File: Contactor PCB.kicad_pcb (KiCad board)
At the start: 2 copper layers, 140.5 x 83.8 mm, 29 parts, among them J1 TSCU, J10 COIL2_CONNECTOR, J11 AUX2_CONNECTOR, J2 TSCU, J3 IMD, J4 AIL, J5 UIL, J6 TBD, J7 COIL_INPUTS, J8 COIL1_CONNECTOR, J9 AUX1_CONNECTOR, U1 Gigavac_GX21CAB, U2 Gigavac_GX21CAB

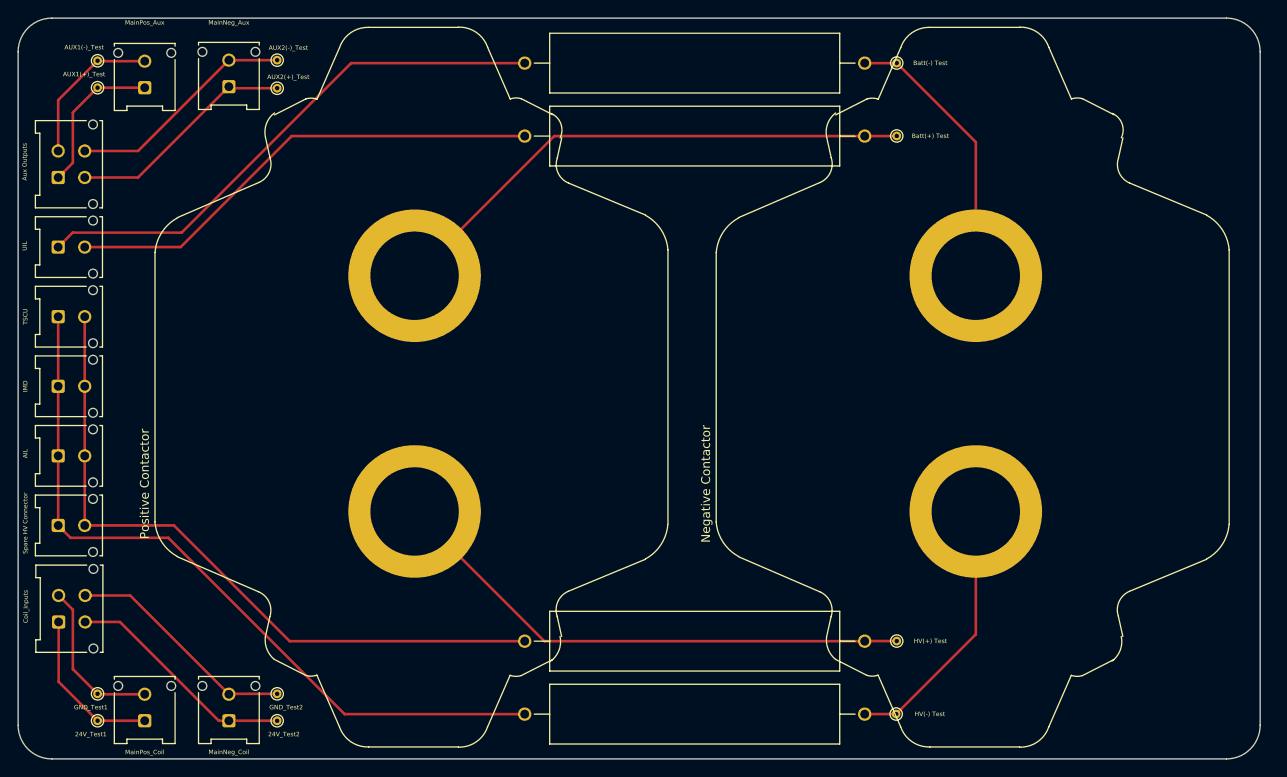
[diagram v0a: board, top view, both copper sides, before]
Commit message: Finalize Board
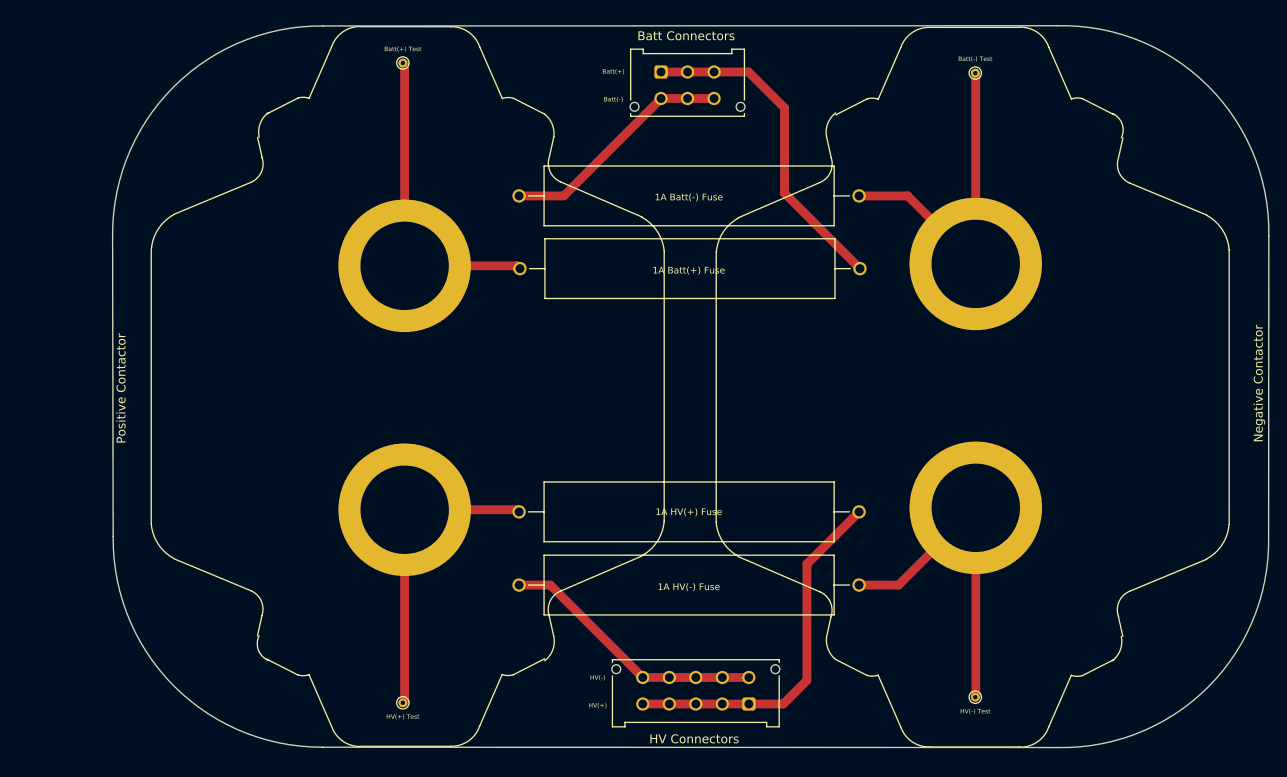
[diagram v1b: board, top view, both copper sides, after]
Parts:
- removed J10: COIL2_CONNECTOR, Connector_Molex:Molex_Micro-Fit_3.0_43045-0212_2x01_P3.00mm_Vertical
- removed J11: AUX2_CONNECTOR, Connector_Molex:Molex_Micro-Fit_3.0_43045-0212_2x01_P3.00mm_Vertical
- removed J3: IMD, Connector_Molex:Molex_Micro-Fit_3.0_43045-0212_2x01_P3.00mm_Vertical
- removed J4: AIL, Connector_Molex:Molex_Micro-Fit_3.0_43045-0212_2x01_P3.00mm_Vertical
- removed J5: UIL, Connector_Molex:Molex_Micro-Fit_3.0_43045-0212_2x01_P3.00mm_Vertical
- removed J6: TBD, Connector_Molex:Molex_Micro-Fit_3.0_43045-0212_2x01_P3.00mm_Vertical
- removed J7: COIL_INPUTS, Connector_Molex:Molex_Micro-Fit_3.0_43045-0412_2x02_P3.00mm_Vertical
- removed J8: COIL1_CONNECTOR, Connector_Molex:Molex_Micro-Fit_3.0_43045-0212_2x01_P3.00mm_Vertical
- removed J9: AUX1_CONNECTOR, Connector_Molex:Molex_Micro-Fit_3.0_43045-0212_2x01_P3.00mm_Vertical
- removed TP10: 24V_TEST2, TestPoint:TestPoint_THTPad_D1.0mm_Drill0.5mm
- removed TP11: GND_TEST1, TestPoint:TestPoint_THTPad_D1.0mm_Drill0.5mm
- removed TP12: 24V_TEST1, TestPoint:TestPoint_THTPad_D1.0mm_Drill0.5mm
- removed TP2, TP6: AUX_TEST(+), TestPoint:TestPoint_THTPad_D1.0mm_Drill0.5mm
- removed TP3, TP7: AUX_TEST(-), TestPoint:TestPoint_THTPad_D1.0mm_Drill0.5mm
- removed TP9: GND_TEST2, TestPoint:TestPoint_THTPad_D1.0mm_Drill0.5mm
- F1, F2, F3, F4: footprint CustomFootprints:Fuse_Placeholder -> CustomFootprints:0ADAP1000RE
- J1: value TSCU -> HV Connector; footprint Connector_Molex:Molex_Micro-Fit_3.0_43045-0212_2x01_P3.00mm_Vertical -> Connector_Molex:Molex_Micro-Fit_3.0_43045-1012_2x05_P3.00mm_Vertical
- J2: value TSCU -> Batt Connector; footprint Connector_Molex:Molex_Micro-Fit_3.0_43045-0412_2x02_P3.00mm_Vertical -> Connector_Molex:Molex_Micro-Fit_3.0_43045-0612_2x03_P3.00mm_Vertical
- moved U1 100.1 mm to (176.9, 44.0), turned to -90 degrees
- moved J1 89.6 mm to (186.5, 120.8), turned to 180 degrees
- moved J2 69.2 mm to (176.5, 49.3), turned to 0 degrees
- moved TP1 56.5 mm to (147.3, 48.3)
- moved TP4 56.3 mm to (147.3, 120.7)
- moved F2 29.0 mm to (179.6, 91.9), turned to 0 degrees
- moved F3 15.0 mm to (179.8, 70.5)
- moved F4 14.6 mm to (179.8, 114.5)
- moved TP8 9.16 mm to (212.1, 120.0)
- moved TP5 8.96 mm to (212.1, 49.4)
- moved F1 0.96 mm to (179.7, 64.3), turned to 0 degrees
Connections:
- F1 pad 1: Net-(F1-Pad1) -> Net-(U1-Pad1)
- F2 pad 1: Net-(F2-Pad1) -> Net-(TP4-Pad1)
- J1 pad 1: /HV(-) -> /HV(+)
- J2 pad 1: /AUX_1(+) -> /Batt(+)
- J2 pad 2: /AUX_1(-) -> /Batt(+)
- J2 pad 3: /AUX_2(+) -> /Batt(+)
- J2 pad 4: /AUX_2(-) -> /Batt(-)
- TP1 pad 1: Net-(F1-Pad1) -> Net-(U1-Pad1)
- TP4 pad 1: Net-(F2-Pad1) -> Net-(TP4-Pad1)
- U1 pad 1: Net-(F2-Pad1) -> Net-(U1-Pad1)
- U1 pad 2: Net-(F1-Pad1) -> Net-(TP4-Pad1)
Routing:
- net Net-(F1-Pad1): track 61.1 -> 0.00 mm
- net Net-(F2-Pad1): track 60.6 -> 0.00 mm
- net /HV(-): track 85.2 -> 30.3 mm
- net /HV(+): track 78.8 -> 41.2 mm
- net Net-(U1-Pad1): track 0.00 -> 36.2 mm
- net Net-(TP4-Pad1): track 0.00 -> 35.0 mm
- net /Batt(-): track 61.4 -> 26.6 mm
- net /GND_2: track 26.4 -> 0.00 mm
- net /24V_IN2: track 26.4 -> 0.00 mm
- net /AUX_2(+): track 26.1 -> 0.00 mm
- net /AUX_2(-): track 26.0 -> 0.00 mm
- net /24V_IN1: track 18.3 -> 0.00 mm
- net /GND_1: track 18.3 -> 0.00 mm
- net /Batt(+): track 55.0 -> 37.4 mm
- net /AUX_1(-): track 17.4 -> 0.00 mm
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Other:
- board size 140.5 x 83.8 mm -> 130.8 x 81.7 mm
- board text added: "1A Batt(+) Fuse"
- board text added: "1A Batt(-) Fuse"
- board text added: "1A HV(+) Fuse"
- board text added: "1A HV(-) Fuse"
- board text added: "Batt Connectors"
- board text added: "Batt(+)"
- board text added: "Batt(-)"
- board text added: "HV Connectors"
- board text added: "HV(+)"
- board text added: "HV(-)"
- board text removed: "24V_Test1"
- board text removed: "24V_Test2"
- board text removed: "AIL"
- board text removed: "AUX1(+)_Test"
- board text removed: "AUX1(-)_Test"
- board text removed: "AUX2(+)_Test"
- board text removed: "AUX2(-)_Test"
- board text removed: "Aux Outputs"
- board text removed: "Coil_Inputs"
- board text removed: "GND_Test1"
- board text removed: "GND_Test2"
- board text removed: "IMD"
- board text removed: "MainNeg_Aux"
- board text removed: "MainNeg_Coil"
- board text removed: "MainPos_Aux"
- board text removed: "MainPos_Coil"
- board text removed: "Spare HV Connector"
- board text removed: "TSCU"
- board text removed: "UIL"
